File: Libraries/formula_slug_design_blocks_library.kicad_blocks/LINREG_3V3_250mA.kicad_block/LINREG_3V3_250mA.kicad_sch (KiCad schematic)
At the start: 3 parts

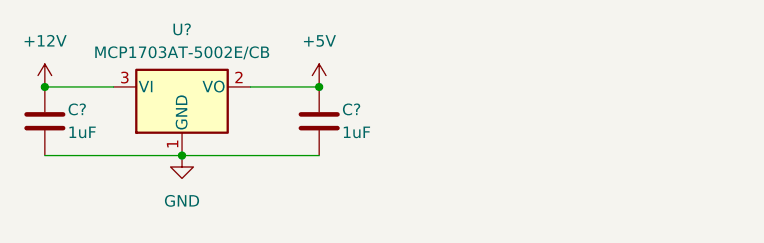
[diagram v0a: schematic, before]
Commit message: fixed 5V linear regulator and added 12->3.3V one
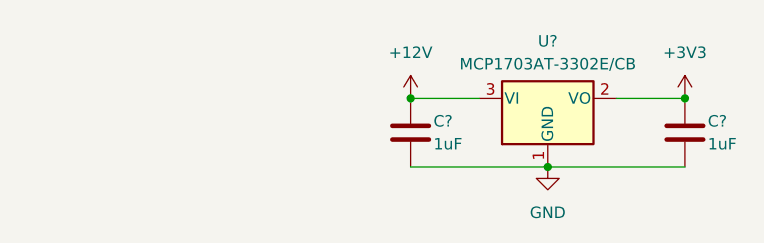
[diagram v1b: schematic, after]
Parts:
- removed C? (x2): 1uF, Capacitor_SMD:C_0603_1608Metric_Pad1.08x0.95mm_HandSolder, symbol Device:C
- removed U?: MCP1703AT-5002E/CB, Package_TO_SOT_SMD:TSOT-23_HandSoldering, symbol Regulator_Linear:MCP1703Ax-500xxTT
- added C? (x2): 1uF, Capacitor_SMD:C_0603_1608Metric_Pad1.08x0.95mm_HandSolder, symbol Device:C
- added U?: MCP1703AT-3302E/CB, Package_TO_SOT_SMD:TSOT-23_HandSoldering, symbol Regulator_Linear:MCP1703Ax-500xxTT
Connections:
- net +12V: now also C?.2, U?.3 (VI)
- net GND: now also C?.1, C?.1, U?.1 (GND)
- new net +3V3: C?.2, U?.2 (VO)

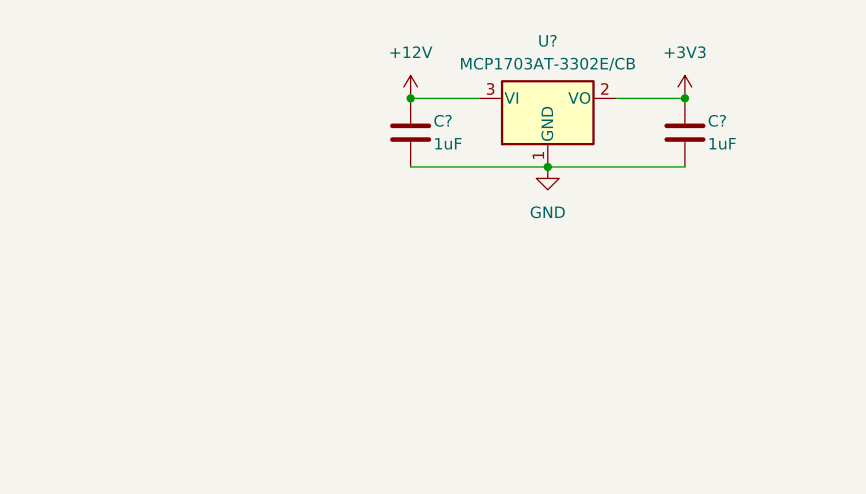
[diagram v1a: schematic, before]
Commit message: Fixed cap digi url links
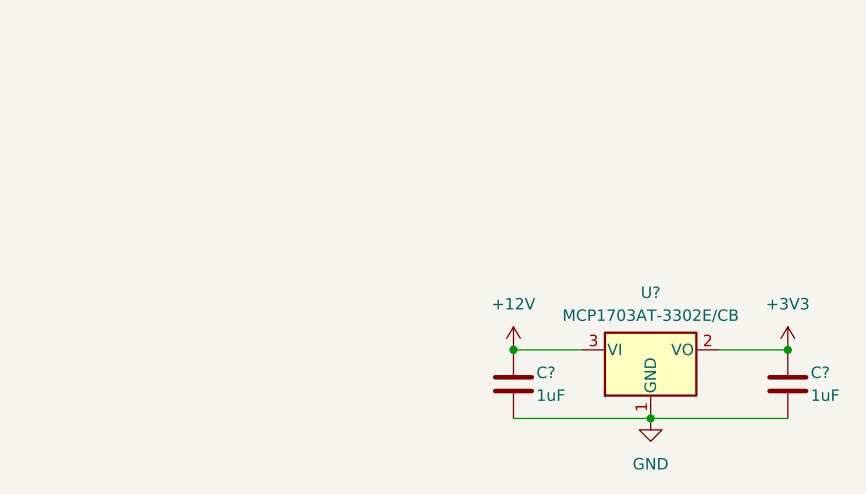
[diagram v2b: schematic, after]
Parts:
- C? (x2): Digi URL (none) -> https://www.digikey.com/en/products/detail/samsung-electro-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
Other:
- moved on the sheet: C?, U?
